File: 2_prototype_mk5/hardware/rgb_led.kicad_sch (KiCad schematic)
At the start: 2 parts

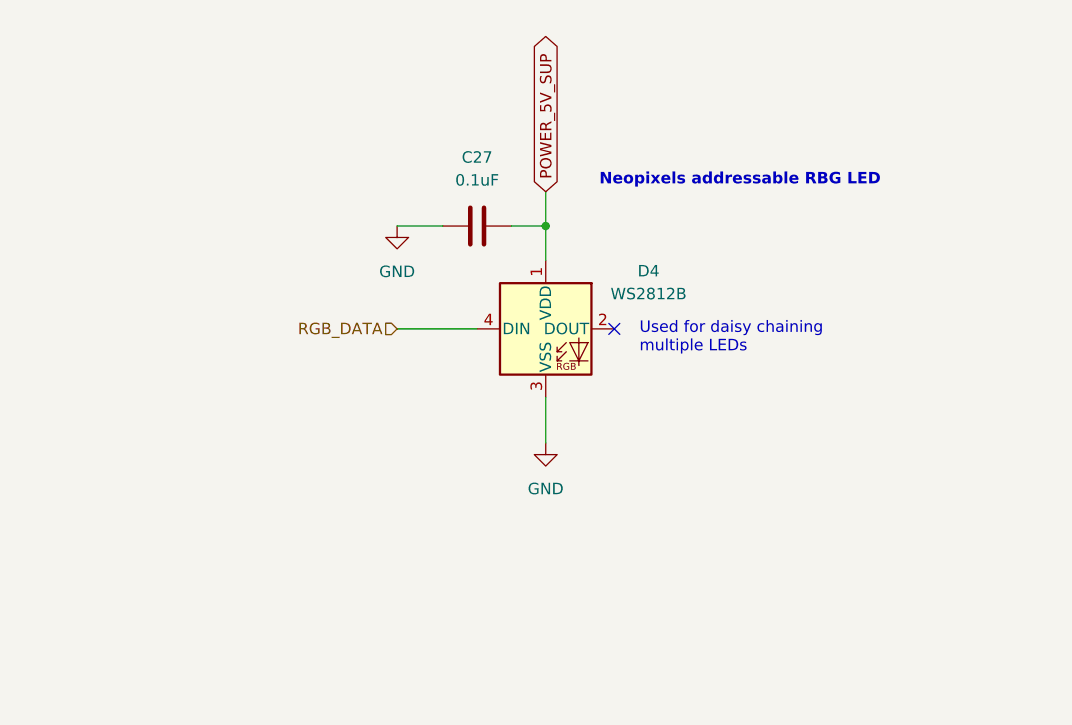
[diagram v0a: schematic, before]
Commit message: MKV revision 1
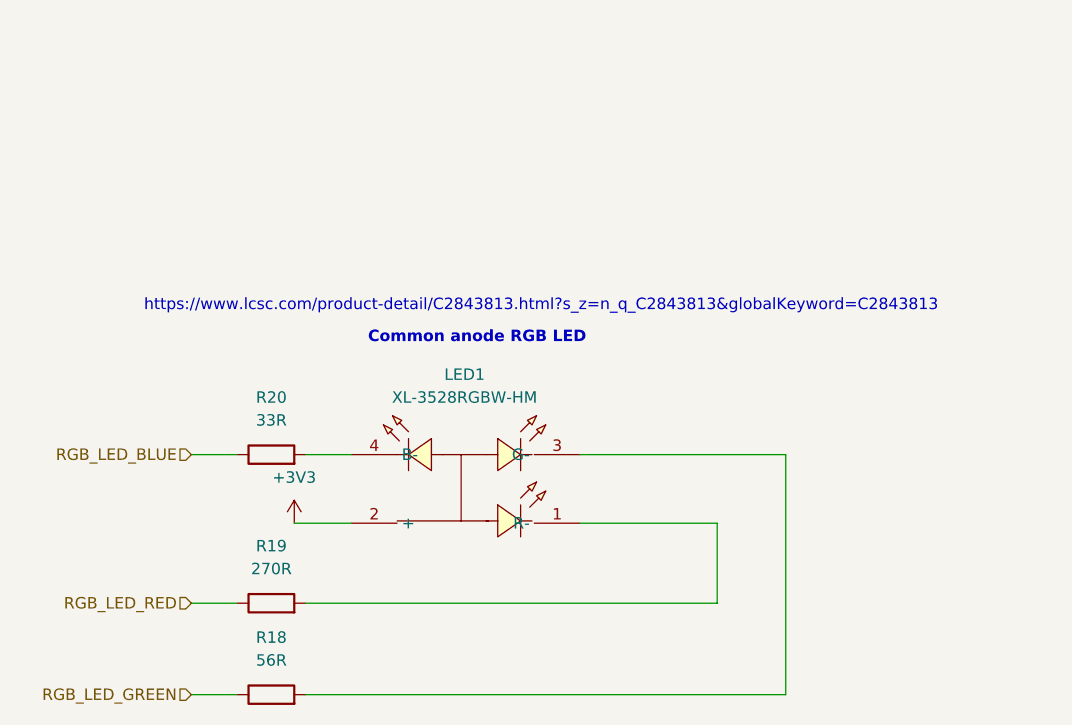
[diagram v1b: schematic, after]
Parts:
- removed C27: 0.1uF, Capacitor_SMD:C_0603_1608Metric, symbol Device:C
- removed D4: WS2812B, LED_SMD:LED_WS2812B_PLCC4_5.0x5.0mm_P3.2mm, symbol LED:WS2812B
- added LED1: XL-3528RGBW-HM, Custom:LED-SMD_4P-L3.2-W2.8-LS3.5-XL-3528RGBW-HM5, symbol Project symbols:XL-3528RGBW-HM
- added R18: 56R, Resistor_SMD:R_0402_1005Metric, symbol Device:R
- added R19: 270R, Resistor_SMD:R_0402_1005Metric, symbol Device:R
- added R20: 33R, Resistor_SMD:R_0402_1005Metric, symbol Device:R
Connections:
- new net: LED1.3 (G-), R18.2
- new net: LED1.1 (R-), R19.2
- new net: LED1.4 (B-), R20.2
- new net +3V3: LED1.2 (+)
- new net RGB_LED_BLUE: R20.1
- new net RGB_LED_GREEN: R18.1
- new net RGB_LED_RED: R19.1
- no-connect marks 1 -> 0
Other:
- note added: "Common anode RGB LED"
- note added: "https://www.lcsc.com/product-detail/C2843813.html?s_z=n_q_C2843813&globalKeyword=C2843813"
- note removed: "Neopixels addressable RBG LED"
- note removed: "Used for daisy chaining multiple LEDs"
